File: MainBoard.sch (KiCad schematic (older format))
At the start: 12 parts

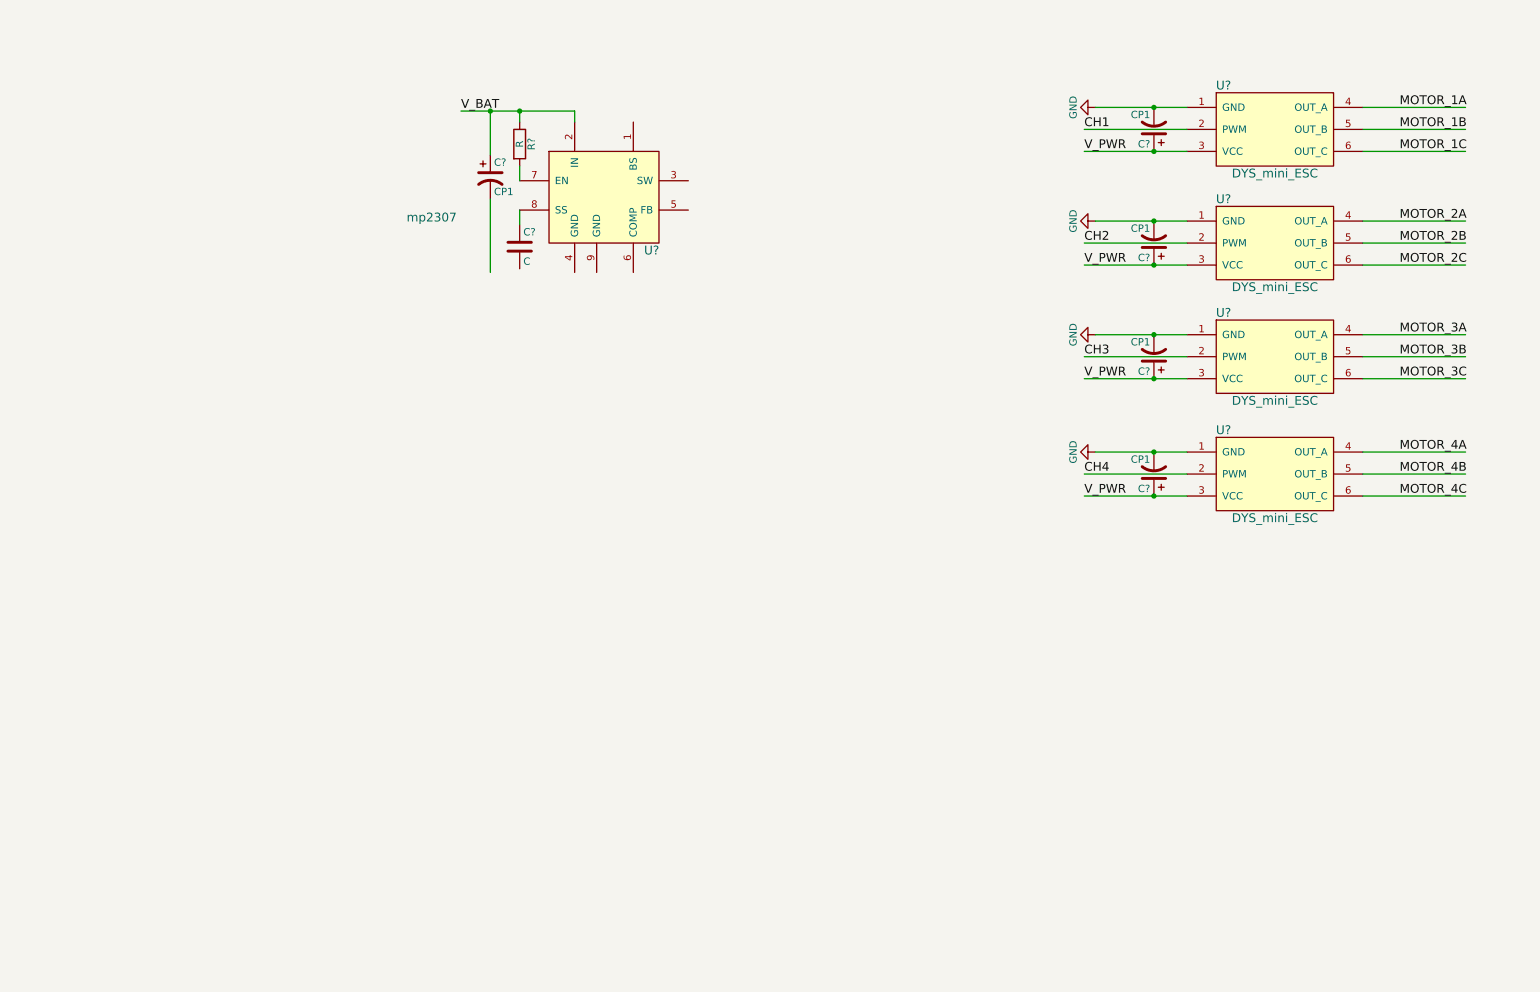
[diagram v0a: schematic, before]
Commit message: main board update
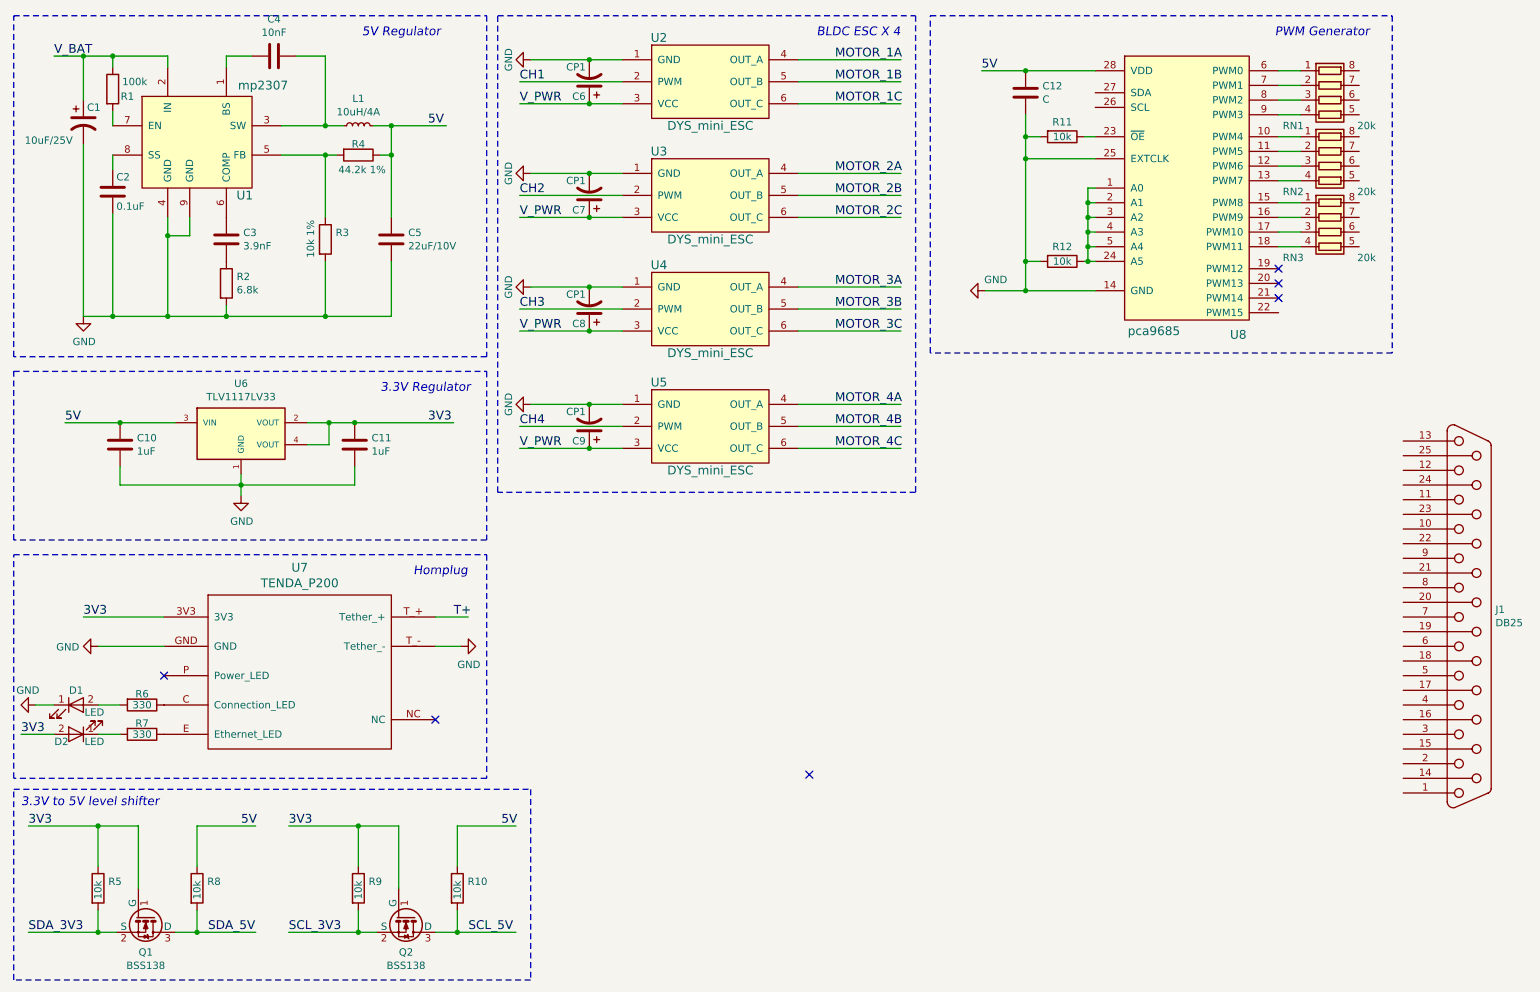
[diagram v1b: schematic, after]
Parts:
- added C10, C11: 1uF, Capacitors_SMD:C_0805, symbol C
- added C12: C, Capacitors_SMD:C_0603, symbol C
- added C3: 3.9nF, Capacitors_SMD:C_0603, symbol C
- added C4: 10nF, Capacitors_SMD:C_0603, symbol C
- added C5: 22uF/10V, Capacitors_SMD:C_0805, symbol C
- added D1, D2: LED, LEDs:LED_0805, symbol LED
- added J1: DB25, Connect:DB25FC, symbol DB25
- added L1: 10uH/4A, footprint:ASPI-0630LR, symbol L_Small
- added Q1, Q2: BSS138, TO_SOT_Packages_SMD:SOT-23, symbol BSS138
- added R10, R11, R12, R5, R8, R9: 10k, Capacitors_SMD:C_0603, symbol R
- added R2: 6.8k, Capacitors_SMD:C_0603, symbol R
- added R3: 10k 1%, Capacitors_SMD:C_0603, symbol R
- added R4: 44.2k 1%, Capacitors_SMD:C_0603, symbol R
- added R6, R7: 330, Capacitors_SMD:C_0603, symbol R
- added RN1, RN2, RN3: 20k, Resistors_SMD:R_Array_Concave_4x0603, symbol R_Pack04
- added U6: TLV1117LV33, TO_SOT_Packages_SMD:SOT-223, symbol TLV1117LV33
- added U7: TENDA_P200, footprint:Tenda_p200, symbol TENDA_P200
- added U8: pca9685, Housings_SSOP:TSSOP-28_4.4x9.7mm_Pitch0.65mm, symbol pca9685
- C1: renamed from C?; value CP1 -> 10uF/25V; footprint (none) -> Capacitors_SMD:C_1206; Part # (none) -> 445-8867-1-ND; Vender (none) -> DigiKey
- C2: renamed from C?; value C -> 0.1uF; footprint (none) -> Capacitors_SMD:C_0603
- R1: renamed from R?; value R -> 100k; footprint (none) -> Capacitors_SMD:C_0603
- U1: renamed from U?; footprint (none) -> Housings_SOIC:SOIC-8-1EP_3.9x4.9mm_Pitch1.27mm; Part # (none) -> 946-MP2307DNLF; Vender (none) -> Mouser
- gave numbers to parts that had none: 8
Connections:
- net labels added: 3V3, 5V, SCL_3V3, SCL_5V, SDA_3V3, SDA_5V, T+
- wire segments 31 -> 109
- no-connect marks 0 -> 6
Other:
- note added: "3.3V Regulator"
- note added: "3.3V to 5V level shifter"
- note added: "5V Regulator"
- note added: "BLDC ESC X 4"
- note added: "Homplug"
- note added: "PWM Generator"
- moved on the sheet: C1, C2, C6, C7, C8, C9, R1, U1, U2, U3, U4, U5
